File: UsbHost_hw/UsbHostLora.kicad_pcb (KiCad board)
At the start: 2 copper layers, 27.2 x 86 mm, 79 parts, among them Q1 LED_RGB 5050

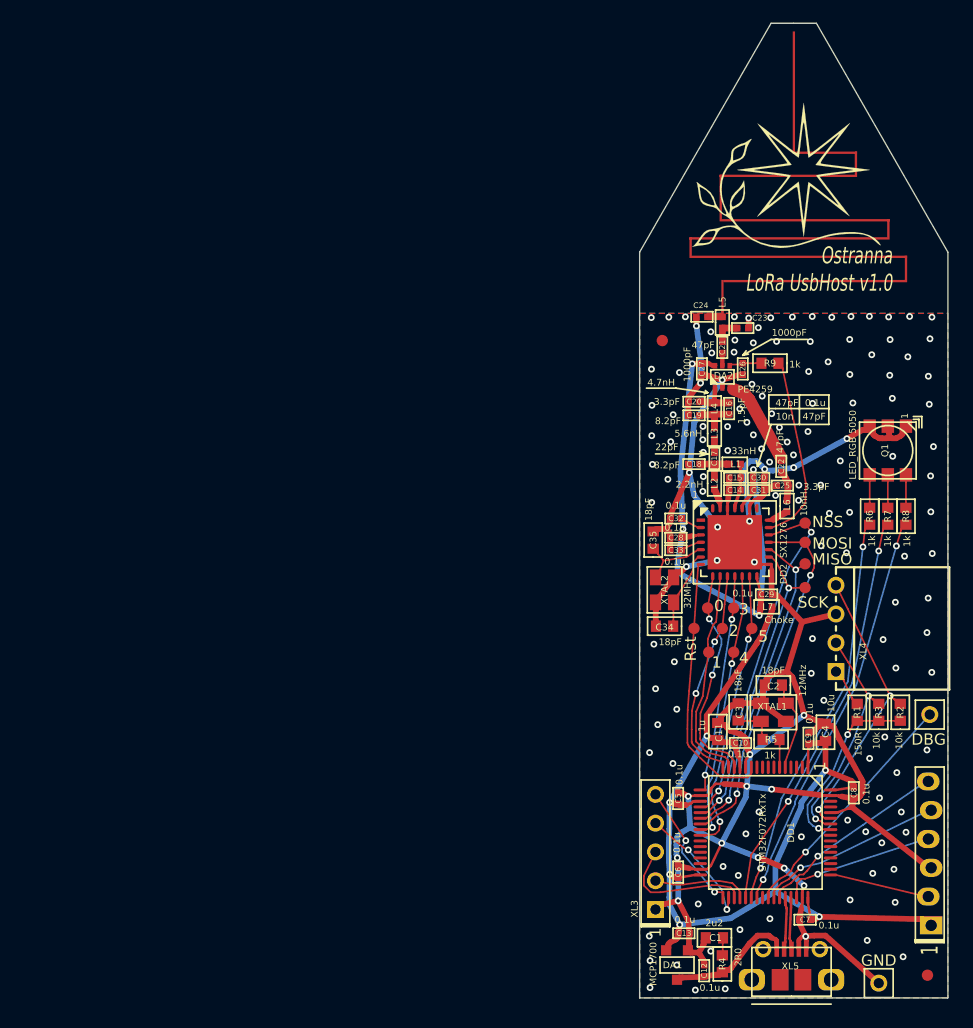
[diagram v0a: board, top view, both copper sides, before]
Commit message: Sent to factory
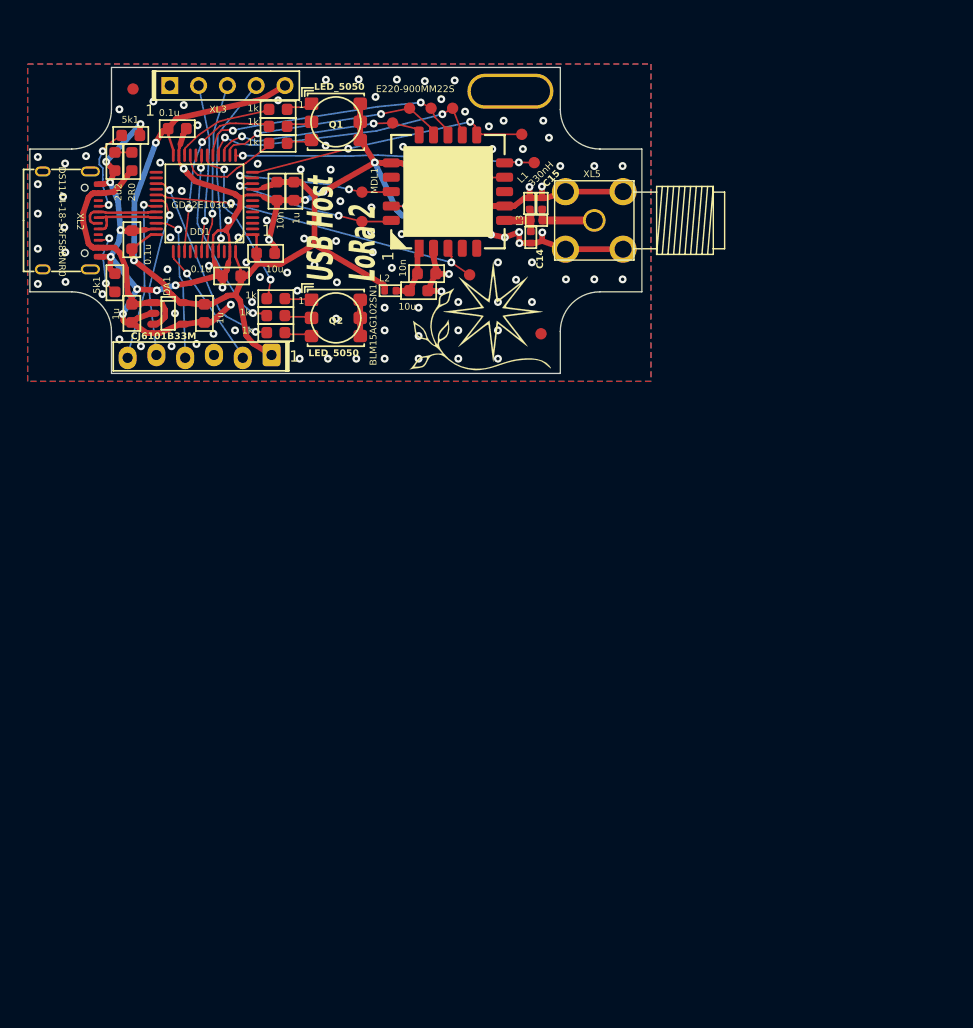
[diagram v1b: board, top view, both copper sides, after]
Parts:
- removed ANT1: ANT_PCB_MONO_2PIN, Antennas:Firefly_868
- removed C10, C28, C29, C30, C32, C33: 0.1u, Capacitors:CAP_0402
- removed C11: 1u, Capacitors:CAP_0603
- removed C16: 1.5pF, Capacitors:CAP_0402
- removed C17: 22pF, Capacitors:CAP_0402
- removed C18, C19: 8.2pF, Capacitors:CAP_0402
- removed C20, C25: 3.3pF, Capacitors:CAP_0402
- removed C21, C22, C31: 47pF, Capacitors:CAP_0402
- removed C23, C24: C, Capacitors:CAP_0402
- removed C26, C27: 1000pF, Capacitors:CAP_0402
- removed C34, C35: 18pF, Capacitors:CAP_0603
- removed DA2: PE4259, SOT:SC70
- removed DD2: SX1276, QFN_DFN:QFN-28_EP_6x6_Pitch0.65mm
- removed L4: 4.7nH, Inductors:IND_0402
- removed L5: L, Inductors:IND_0402
- removed L6: 10nH, Inductors:IND_0402
- removed L7: Choke, Inductors:IND_0402
- removed TP10, TP11: TESTPOINT, PCB:TESTPOINT_1MM
- removed XL6: CONN_1, Connectors:PLS-1Rnd
- removed XTAL1: 12MHz, Quartz:03225C4
- removed XTAL2: 32MHz, Quartz:03225C4
- added MDL1: E220-900MM22S, Modules:E220-900MM22S, F.Cu at (125.1, 70.3)
- added Q2: LED_5050, LEDs:LED_5050, F.Cu at (115.2, 81.4)
- C1: value 2u2 -> 1u; footprint Capacitors:CAP_0603 -> Capacitors:CAP_0603_Silks
- C12, C5: value 0.1u -> 10n; footprint Capacitors:CAP_0402 -> Capacitors:CAP_0603_Silks
- C13, C6: value 0.1u -> 10u; footprint Capacitors:CAP_0402 -> Capacitors:CAP_0603_Silks
- C14: value 10n -> DNM; footprint Capacitors:CAP_0402 -> Capacitors:CAP_0402_Silks
- C15: value 47pF -> DNM; footprint Capacitors:CAP_0402 -> Capacitors:CAP_0402_Silks
- C2: value 18pF -> 2u2; footprint Capacitors:CAP_0603 -> Capacitors:CAP_0603_Silks
- C3: value 18pF -> 1u; footprint Capacitors:CAP_0603 -> Capacitors:CAP_0603_Silks
- C4: value 10u -> 1u; footprint Capacitors:CAP_0603 -> Capacitors:CAP_0603_Silks
- C7, C8, C9: footprint Capacitors:CAP_0402 -> Capacitors:CAP_0603_Silks
- DA1: value MCP1700 -> CJ6101B33M; footprint SOT:SOT23-3A -> SOT:SOT23-5
- DD1: value STM32F072RxTx -> GD32E103CB; footprint LQFP_TQFP:LQFP64 -> LQFP_TQFP:LQFP48
- L1: value 33nH -> 330nH
- L2: value 2.2nH -> BLM15AG102SN1
- L3: value 5.6nH -> 0R
- Logo1: footprint Pictures:Ostranna_16d9_13d5 -> Pictures:Ostranna_12d7_10d1
- Q1: value LED_RGB 5050 -> LED_5050
- R1: value 150R -> 2R0; footprint Resistors:RES_0603 -> Resistors:RES_0603_RefFab
- R2, R3: value 10k -> 5k1; footprint Resistors:RES_0603 -> Resistors:RES_0603_RefFab
- R4: value 2R0 -> 1k; footprint Resistors:RES_0603 -> Resistors:RES_0603_RefFab
- R5, R6, R7, R8, R9: footprint Resistors:RES_0603 -> Resistors:RES_0603_RefFab
- XL1: value CONN_6 -> SOCKET_6
- XL2: value CONN_1 -> DS1144-18-16FS8BNR0; footprint Connectors:PLS-1Rnd -> Connectors:USBC_10PF-074_1
- XL3: value CONN_5 -> SOCKET_5
- XL4: value CONN_4 -> CONN_1; footprint Connectors:PBS-4R -> PCB:OSCIL_GND
- XL5: value USB_MICRO_2H -> SMA_L; footprint Connectors:USBmicro_MOLEX_1050170001 -> Connectors:SMA_R
- moved RP1 105.0 mm to (97.3, 61.2)
- moved C7 89.1 mm to (101.2, 64.7), turned to 0 degrees
- moved XL2 85.9 mm to (93.5, 72.8), turned to -90 degrees
- moved R4 85.0 mm to (110.1, 63.0), turned to 0 degrees
- moved R2 84.9 mm to (97.1, 65.3), turned to 180 degrees
- moved XL3 84.4 mm to (100.5, 60.9), turned to 0 degrees
- moved R1 80.4 mm to (97.2, 67.6)
- moved C8 80.2 mm to (97.2, 74.5), turned to 90 degrees
- moved R3 77.3 mm to (95.7, 78.3)
- moved XL1 76.8 mm to (109.5, 84.8), turned to 180 degrees
- moved C1 75.4 mm to (97.2, 81.0), turned to -90 degrees
- moved DD1 74.4 mm to (103.6, 71.3), turned to 180 degrees
- moved C2 74.2 mm to (95.7, 67.6), turned to -90 degrees
- moved DA1 73.0 mm to (100.4, 81.0), turned to -90 degrees
- moved XL5 70.6 mm to (138.0, 72.8)
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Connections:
- C1 pad 1: Net-(C1-Pad1) -> +5vUSB
- C12 pad 1: /5V_USB -> /+R_PWR
- C13 pad 1: +3v3 -> /+R_PWR
- C14 pad 1: Net-(C14-Pad1) -> /ANT3
- C15 pad 1: Net-(C14-Pad1) -> Net-(C15-Pad1)
- C3 pad 1: Net-(C3-Pad1) -> +3v3
- DA1 pad 1: GND -> +5vUSB
- DA1 pad 2: +3v3 -> GND
- DA1 pad 3: /5V_USB -> +5vUSB
- DD1 pad 10: unconnected-(DD1-Pad10) -> /R_DIO1
- DD1 pad 11: /SX_RST -> /R_DIO3
- DD1 pad 12: GND -> /R_BUSY
- DD1 pad 13: +3v3 -> /R_RXEN
- DD1 pad 14: /SX_DIO0 -> /R_NSS
- DD1 pad 15: /SX_DIO1 -> /R_SCK
- DD1 pad 16: /SX_DIO2 -> /R_MISO
- DD1 pad 17: /SX_DIO3 -> /R_MOSI
- DD1 pad 18: GND -> /LED2_B
- DD1 pad 19: +3v3 -> /LED2_R
- DD1 pad 20: /SX_NSS -> unconnected-(DD1-PB2-Pad20)
- DD1 pad 21: /SX_SCK -> /LED1_G
- DD1 pad 22: /SX_MISO -> /LED1_B
- DD1 pad 23: /SX_MOSI -> GND
- DD1 pad 24: /SX_DIO4 -> +3v3
- DD1 pad 25: /SX_DIO5 -> unconnected-(DD1-PB12-Pad25)
- DD1 pad 27: unconnected-(DD1-Pad27) -> /LED2_G
- DD1 pad 29: unconnected-(DD1-Pad29) -> /R_RST
- DD1 pad 30: unconnected-(DD1-Pad30) -> /UART_TX
- DD1 pad 31: GND -> /UART_RX
- DD1 pad 32: +3v3 -> /USB.DN
- DD1 pad 33: Net-(DD1-Pad33) -> /USB.DP
- DD1 pad 34: Net-(DD1-Pad34) -> /SWDIO
- DD1 pad 35: Net-(DD1-Pad35) -> GND
- DD1 pad 36: Net-(DD1-Pad36) -> +3v3
- DD1 pad 37: /RED_LED -> /SWCLK
- DD1 pad 38: /GREEN_LED -> unconnected-(DD1-JTDI-Pad38)
- DD1 pad 39: /BLUE_LED -> /LED1_R
- DD1 pad 41: Net-(DD1-Pad41) -> unconnected-(DD1-PB5-Pad41)
- DD1 pad 42: /UART_TX -> /PB6
- DD1 pad 43: /UART_RX -> /PB7
- DD1 pad 44: /USB_D- -> GND
- DD1 pad 45: /USB_D+ -> /PB8
- DD1 pad 46: /SWDIO -> unconnected-(DD1-PB9-Pad46)
- DD1 pad 5: Net-(C2-Pad1) -> unconnected-(DD1-OSCIN-Pad5)
- DD1 pad 6: Net-(DD1-Pad6) -> unconnected-(DD1-OSCOUT-Pad6)
- DD1 pad 8: unconnected-(DD1-Pad8) -> GND
- DD1 pad 9: unconnected-(DD1-Pad9) -> +3v3
- L1 pad 1: Net-(C14-Pad1) -> GND
- L1 pad 2: Net-(C17-Pad2) -> /ANT3
- L2 pad 1: Net-(DD2-Pad27) -> +3v3
- L2 pad 2: Net-(C17-Pad2) -> /+R_PWR
- L3 pad 1: Net-(C17-Pad1) -> Net-(C15-Pad1)
- L3 pad 2: Net-(C16-Pad2) -> /ANT3
- Q1 pad 1: GND -> Net-(Q1-Pad1)
- Q1 pad 2: GND -> Net-(Q1-Pad2)
- Q1 pad 3: GND -> Net-(Q1-Pad3)
- Q1 pad 4: Net-(Q1-Pad4) -> GND
- Q1 pad 5: Net-(Q1-Pad5) -> GND
- Q1 pad 6: Net-(Q1-Pad6) -> GND
- R1 pad 1: /PWR_PILL -> +5vUSB
- R1 pad 2: /PWR_PILL_PROT -> Net-(C2-Pad1)
- R2 pad 1: /PWR_PILL -> GND
- R2 pad 2: /SDA_PILL -> Net-(XL2-CC1)
- R3 pad 1: /PWR_PILL -> Net-(XL2-CC2)
- R3 pad 2: /SCL_PILL -> GND
- R4 pad 1: /5V_USB -> /LED1_B
- R4 pad 2: Net-(C1-Pad1) -> Net-(Q1-Pad1)
- R5 pad 1: Net-(C3-Pad1) -> /LED1_R
- R5 pad 2: Net-(DD1-Pad6) -> Net-(Q1-Pad2)
- R6 pad 1: /GREEN_LED -> /LED1_G
- R6 pad 2: Net-(Q1-Pad4) -> Net-(Q1-Pad3)
- R7 pad 1: /RED_LED -> /LED2_B
- R7 pad 2: Net-(Q1-Pad5) -> Net-(Q2-Pad1)
- R8 pad 1: /BLUE_LED -> /LED2_R
- R8 pad 2: Net-(Q1-Pad6) -> Net-(Q2-Pad2)
- R9 pad 1: Net-(DD2-Pad20) -> /LED2_G
- RP1 pad REF: (no net) -> unconnected-(RP1-PadREF)
- RP2 pad REF: (no net) -> unconnected-(RP2-PadREF)
- TP1 pad 1: /SX_RST -> /R_DIO1
- TP2 pad 1: /SX_DIO0 -> /R_DIO3
- TP3 pad 1: /SX_DIO1 -> /R_BUSY
- TP4 pad 1: /SX_DIO2 -> /R_RXEN
- TP5 pad 1: /SX_DIO3 -> /R_NSS
- TP6 pad 1: /SX_DIO4 -> /R_SCK
- TP7 pad 1: /SX_DIO5 -> /R_MISO
- TP8 pad 1: /SX_SCK -> /R_MOSI
- TP9 pad 1: /SX_MISO -> /R_RST
- XL3 pad 2: Net-(DD1-Pad36) -> /PB6
- XL3 pad 3: Net-(DD1-Pad35) -> /PB7
- XL3 pad 4: Net-(DD1-Pad34) -> /PB8
- XL3 pad 5: Net-(DD1-Pad33) -> +3v3
- XL4 pad 1: /PWR_PILL_PROT -> GND
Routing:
- net GND: track 247.2 -> 167.1 mm, vias 151 -> 123
- net VCC: track 52.1 -> 0.00 mm, vias 4 -> 0
- net /RED_LED: track 35.8 -> 0.00 mm, vias 2 -> 0
- net /BLUE_LED: track 35.7 -> 0.00 mm, vias 2 -> 0
- net /GREEN_LED: track 35.2 -> 0.00 mm, vias 2 -> 0
- net /SX_MOSI: track 31.3 -> 0.00 mm, vias 2 -> 0
- net /SX_NSS: track 31.1 -> 0.00 mm, vias 2 -> 0
- net /R_RST: track 0.00 -> 30.1 mm, vias 0 -> 2
- net /SX_MISO: track 28.4 -> 0.00 mm, vias 2 -> 0
- net /R_RXEN: track 0.00 -> 27.7 mm, vias 0 -> 2
- net /SX_SCK: track 26.8 -> 0.00 mm, vias 2 -> 0
- net /SDA_PILL: track 25.4 -> 0.00 mm, vias 2 -> 0
- net /R_BUSY: track 0.00 -> 25.1 mm, vias 0 -> 2
- net /R_MISO: track 0.00 -> 24.8 mm, vias 0 -> 2
- net /SX_DIO5: track 24.8 -> 0.00 mm, vias 2 -> 0
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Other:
- board size 27.2 x 86 mm -> 54 x 27 mm
- board text added: "USB Host LoRa 2"
- board text removed: "0"
- board text removed: "1"
- board text removed: "2"
- board text removed: "3"
- board text removed: "4"
- board text removed: "5"
- board text removed: "DBG"
- board text removed: "GND"
- board text removed: "MISO"
- board text removed: "MOSI"
- board text removed: "NSS"
- board text removed: "Ostranna LoRa UsbHost v1.0"
- board text removed: "Rst"
- board text removed: "SCK"
